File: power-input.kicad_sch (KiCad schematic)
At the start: 21 parts, among them J204 Conn_01x02, J301 Conn_01x02, U202 XL1509-3.3

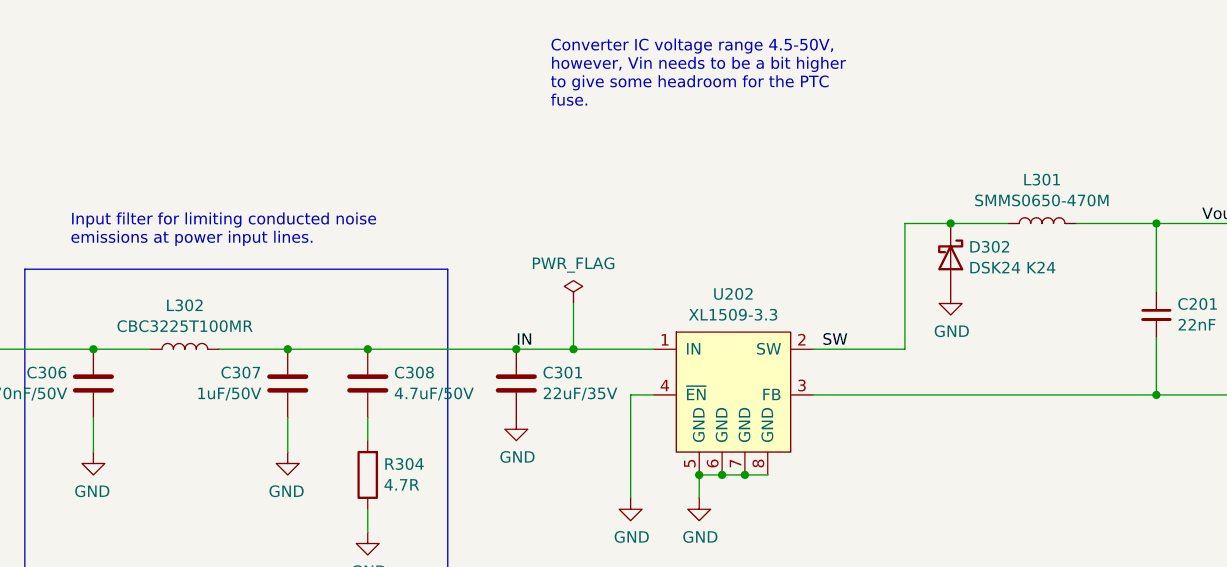
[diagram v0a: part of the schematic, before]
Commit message: Save schema with KiCad 7.0.6
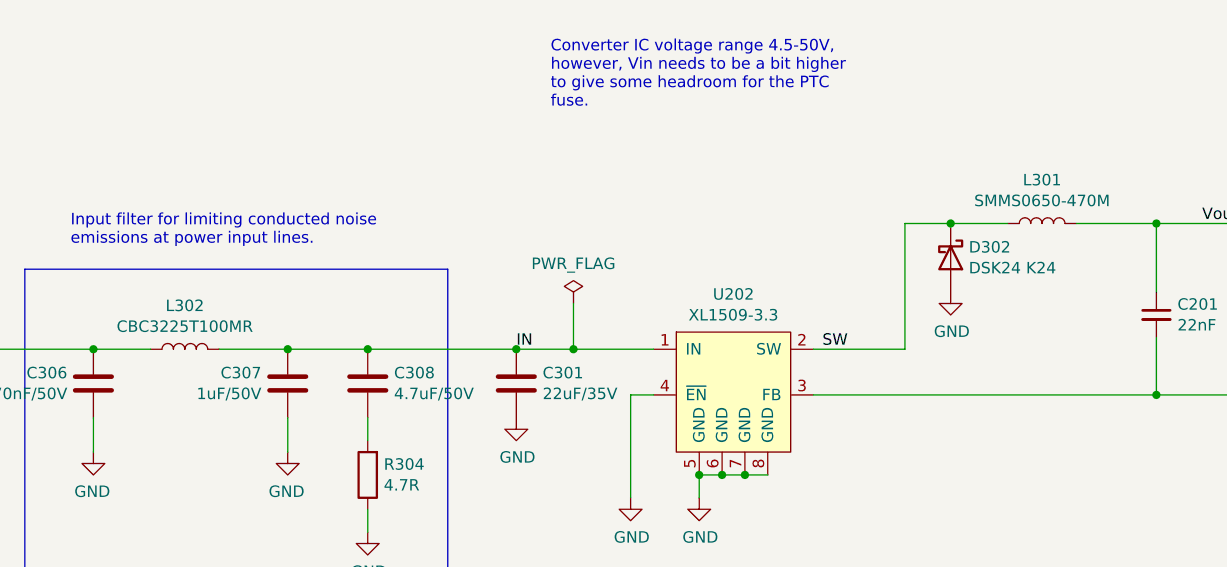
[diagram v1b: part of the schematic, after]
